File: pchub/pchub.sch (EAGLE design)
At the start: 73 parts, among them J6 2040210-1, J7 2040210-1, U1 SN74CBT16214DGGR, U10 FSUSB63UMX, U11 FSUSB63UMX, U12 FSUSB63UMX, U13 FSUSB63UMX, U14 FSUSB63UMX, U15 FSUSB63UMX, U16 FSUSB63UMX, U17 FSUSB63UMX, U18 FSUSB63UMX, U19 FSUSB63UMX, U2 SN74CBT16214DGGR, U20 FSUSB63UMX, U3 SN74CBT16214DGGR, U4 SN74CBT16214DGGR, U5 TMDS361BPAG, U6 TMDS361BPAG, U7 TMDS361BPAG, U8 TMDS361BPAG, U9 FSUSB63UMX, X1 USB, X10 USB, X11 USB, X12 USB, X13 USB, X2 USB, X3 USB, X4 USB, X5 USB, X6 USB, X7 USB, X8 USB, X9 USB

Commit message: m
,
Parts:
- added S17: (no value), SparkFun-Switches:SWITCH-SP3T-SMD
- added U$10, U$11, U$12, U$13, U$14, U$15, U$16, U$17, U$18, U$6, U$7, U$8, U$9: RJ45-8PTH, SparkFun:RJ45-8PTH
- added U21, U22: MAX4998ETIT, MAX4998ETIT:MAX4998ETIT
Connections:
- new net ETH1: U$10.1, U$11.1, U$12.1, U$13.1, U$14.1, U$15.1, U$16.1, U$17.1, U$18.1, U$6.1, U$7.1, U$8.1, U$9.1
- new net ETH2: U$10.2, U$11.2, U$12.2, U$13.2, U$14.2, U$15.2, U$16.2, U$17.2, U$18.2, U$6.2, U$7.2, U$8.2, U$9.2
- new net ETH3: U$10.3, U$11.3, U$12.3, U$13.3, U$14.3, U$15.3, U$16.3, U$17.3, U$18.3, U$6.3, U$7.3, U$8.3, U$9.3
- new net ETH4: U$10.4, U$11.4, U$12.4, U$13.4, U$14.4, U$15.4, U$16.4, U$17.4, U$18.4, U$6.4, U$7.4, U$8.4, U$9.4
- new net ETH5: U$10.5, U$11.5, U$12.5, U$13.5, U$14.5, U$15.5, U$16.5, U$17.5, U$18.5, U$6.5, U$7.5, U$8.5, U$9.5
- new net ETH6: U$10.6, U$11.6, U$12.6, U$13.6, U$14.6, U$15.6, U$16.6, U$17.6, U$18.6, U$6.6, U$7.6, U$8.6, U$9.6
- new net ETH7: U$10.7, U$11.7, U$12.7, U$13.7, U$14.7, U$15.7, U$16.7, U$17.7, U$18.7, U$6.7, U$7.7, U$8.7, U$9.7
- new net ETH8: U$10.8, U$11.8, U$12.8, U$13.8, U$14.8, U$15.8, U$16.8, U$17.8, U$18.8, U$6.8, U$7.8, U$8.8, U$9.8
- net HDMIGND: now also J1SHIELD.SHIELD
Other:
- note added: "ETHERNET"
- moved on the sheet: J1G$1, J1SHIELD, J6, J7

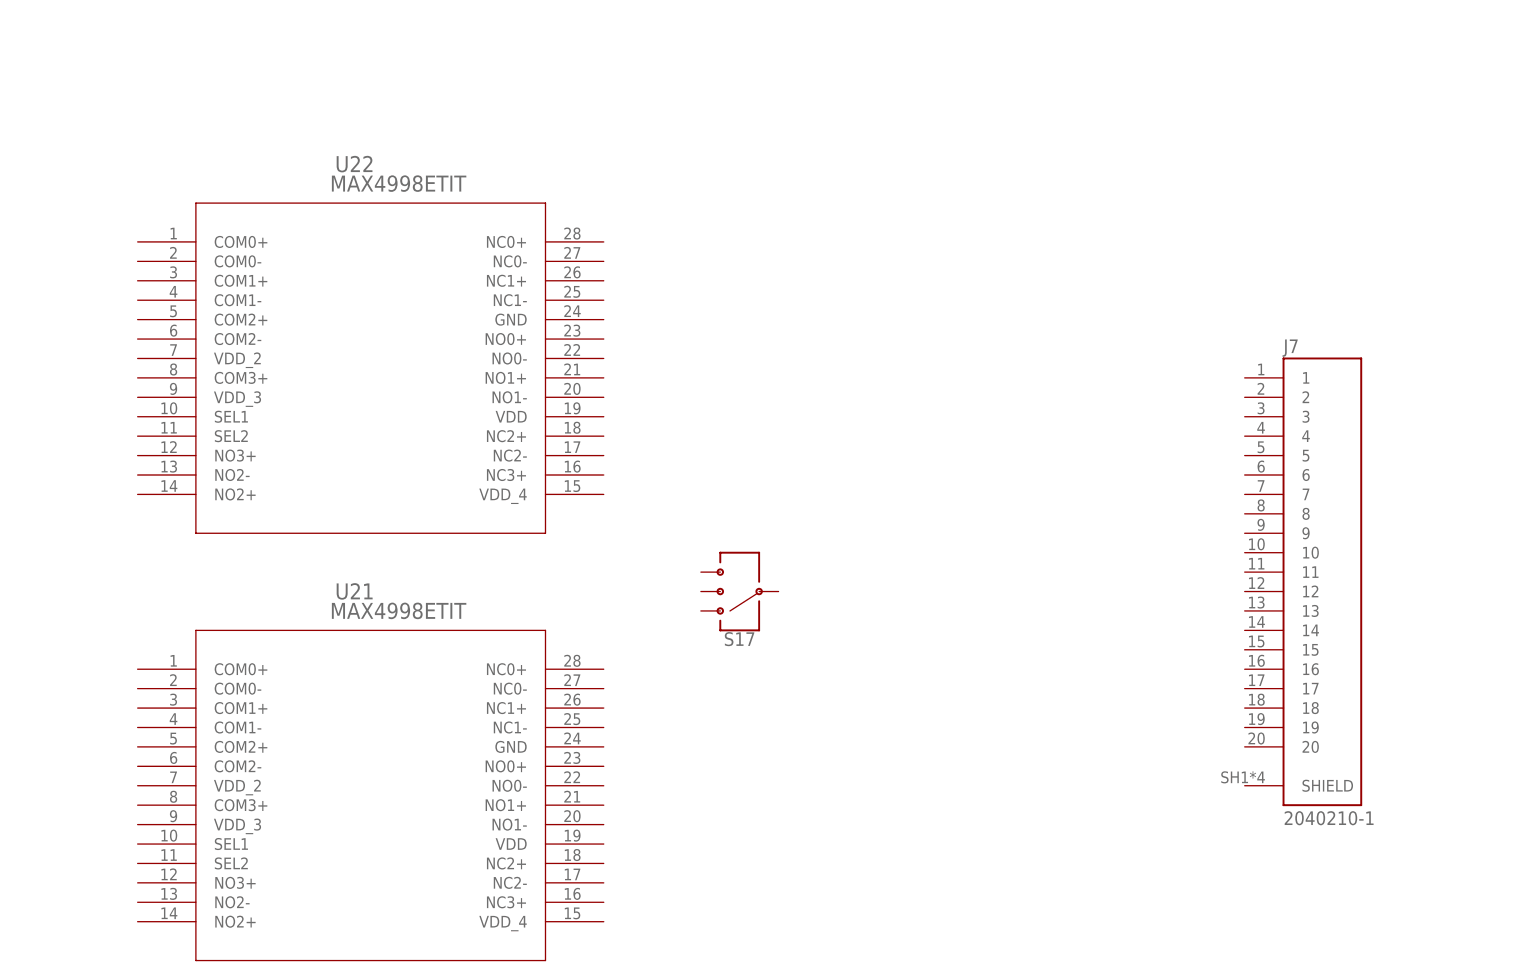
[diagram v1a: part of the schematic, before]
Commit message: sd
asdsa
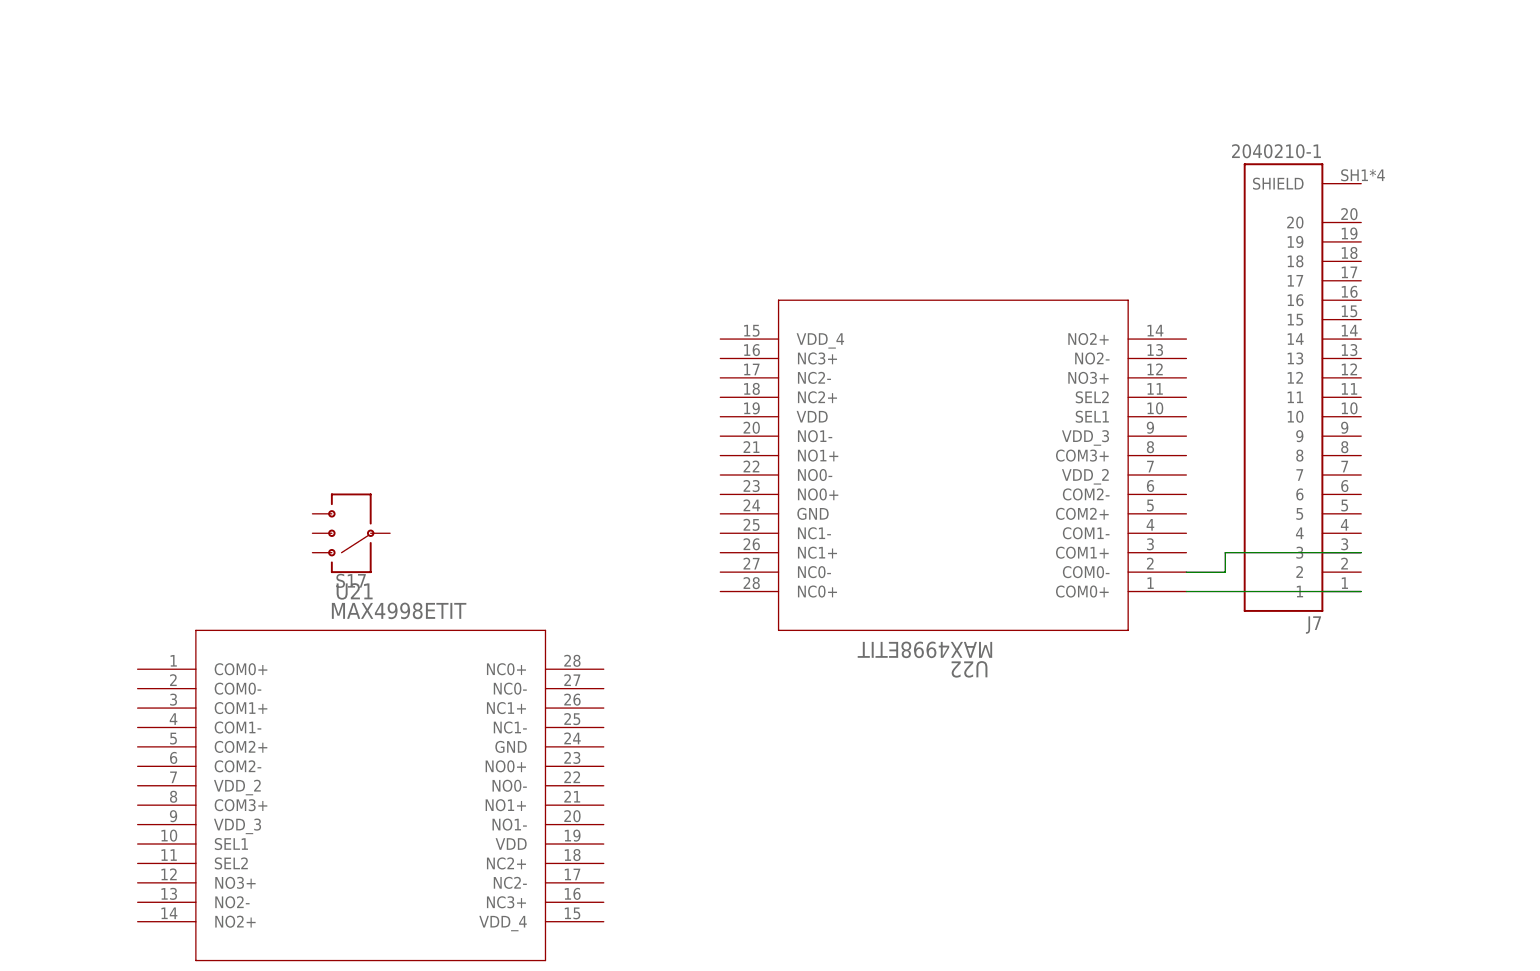
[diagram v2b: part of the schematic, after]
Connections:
- new net N$130: J7.1, U22.COM0+
- new net N$131: J7.3, U22.COM0-
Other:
- moved on the sheet: J7, S17, U22
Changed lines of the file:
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@@
 <layer number="59" name="tCarbon" color="7" fill="1" visible="no" active="no"/>
 <layer number="60" name="bCarbon" color="7" fill="1" visible="no" active="no"/>
-<layer number="88" name="SimResults" color="9" fill="1" visible="yes" active="yes"/>
+<layer number="88" name="SimResults" color="9" fill="1" visible="no" active="yes"/>
 <layer number="89" name="SimProbes" color="9" fill="1" visible="yes" active="yes"/>
 <layer number="90" name="Modules" color="5" fill="1" visible="yes" active="yes"/>
@@
 <instance part="D12" gate="G$1" x="-431.8" y="190.5" rot="R270"/>
 <instance part="J6" gate="G$1" x="-601.98" y="231.14"/>
-<instance part="J7" gate="G$1" x="-213.36" y="-119.38"/>
+<instance part="J7" gate="G$1" x="-218.44" y="-91.44" rot="R180"/>
 <instance part="U$6" gate="G$1" x="-601.98" y="287.02"/>
 <instance part="U$11" gate="G$1" x="-317.5" y="127"/>
@@
 <instance part="U$18" gate="G$1" x="-424.18" y="30.48"/>
 <instance part="U21" gate="A" x="-368.3" y="-129.54"/>
-<instance part="U22" gate="A" x="-368.3" y="-73.66"/>
-<instance part="S17" gate="G$1" x="-289.56" y="-119.38" rot="R180"/>
+<instance part="U22" gate="A" x="-231.14" y="-119.38" rot="R180"/>
+<instance part="S17" gate="G$1" x="-340.36" y="-111.76" rot="R180"/>
 </instances>
 <busses>
@@
 </segment>
 </net>
+<net name="N$130" class="0">
+<segment>
+<pinref part="U22" gate="A" pin="COM0+"/>
+<pinref part="J7" gate="G$1" pin="1"/>
+<wire x1="-231.14" y1="-119.38" x2="-208.28" y2="-119.38" width="0.1524" layer="91"/>
+</segment>
+</net>
+<net name="N$131" class="0">
+<segment>
+<pinref part="J7" gate="G$1" pin="3"/>
+<wire x1="-208.28" y1="-114.3" x2="-226.06" y2="-114.3" width="0.1524" layer="91"/>
+<wire x1="-226.06" y1="-114.3" x2="-226.06" y2="-116.84" width="0.1524" layer="91"/>
+<pinref part="U22" gate="A" pin="COM0-"/>
+<wire x1="-226.06" y1="-116.84" x2="-231.14" y2="-116.84" width="0.1524" layer="91"/>
+</segment>
+</net>

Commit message: s
s
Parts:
- removed U$10, U$11, U$12, U$13, U$14, U$15, U$16, U$17, U$18, U$7, U$8, U$9: RJ45-8PTH, SparkFun:RJ45-8PTH
- added J10, J8, J9: 2040210-1, 2040210-1:2040210-1
- added J11, J12: AUDIO_JACK_TRRSSMD_RA, SparkFun-Connectors:AUDIO_JACK_TRRSSMD_RA
- added S18, S19, S20: (no value), SparkFun-Switches:SWITCH-SP3T-SMD
- added U$19, U$20, U$21, U$22, U$23, U$24, U$25, U$26, U$27, U$28, U$29, U$30: RJ45-8PTH, SparkFun:RJ45-8PTH
- added U23, U24, U25, U26, U27, U28: SN74CBT16214DGGR, SN74CBT16214DGGR:SN74CBT16214DGGR
- U21, U22: value MAX4998ETIT -> SN74CBT16214DGGR; device MAX4998ETIT:MAX4998ETIT -> SN74CBT16214DGGR:SN74CBT16214DGGR
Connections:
- new net B$1: U21.10A, U23.10A, U25.10A, U27.10A
- new net B$2: U21.11A, U23.11A, U25.11A, U27.11A
- new net N$143: J7.3, U21.3A
- new net N$144: J7.4, U21.4A
- new net N$145: J7.5, U21.5A
- new net N$146: J7.6, U21.6A
- new net N$147: J7.7, U21.7A
- new net N$148: J7.8, U21.8A
- new net N$149: J7.9, U21.9A
- new net N$150: J7.10
- new net N$151: J7.11
- new net N$152: J7.12, U21.12A
- new net N$153: J7.13, U22.1A
- new net N$154: J7.14, U22.2A
- new net N$155: J7.15, U22.3A
- new net N$156: J7.16, U22.4A
- new net N$157: J7.17, U22.5A
- new net N$158: J7.18, U22.6A
- new net N$159: J7.19, U22.7A
- new net N$160: J7.SHIELD, U22.9A
- new net N$161: J8.1, U23.1A
- new net N$162: J8.2, U23.2A
- new net N$163: J7.20, U22.8A
- new net N$164: J8.3, U23.3A
- new net N$165: J8.4, U23.4A
- new net N$166: J8.5, U23.5A
- new net N$167: J8.6, U23.6A
- new net N$168: J8.7, U23.7A
- new net N$169: J8.8, U23.8A
- new net N$170: J8.9, U23.9A
- new net N$171: J8.10
- new net N$172: J8.11
- new net N$173: J8.12, U23.12A
- new net N$174: J8.13, U24.1A
- new net N$175: J8.14, U24.2A
- new net N$176: J8.15, U24.3A
- new net N$177: J8.16, U24.4A
- new net N$178: J8.17, U24.5A
- new net N$179: J8.18, U24.6A
- new net N$180: J8.19, U24.7A
- new net N$181: J8.SHIELD, U24.9A
- new net N$182: J8.20, U24.8A
- new net N$183: J9.1, U25.1A
- new net N$184: J9.2, U25.2A
- new net N$185: J9.3, U25.3A
- new net N$186: J9.4, U25.4A
- new net N$187: J9.5, U25.5A
- new net N$188: J9.6, U25.6A
- new net N$189: J9.7, U25.7A
- new net N$190: J9.8, U25.8A
- new net N$191: J9.9, U25.9A
- new net N$192: J9.10
- new net N$193: J9.11
- new net N$194: J9.12, U25.12A
- new net N$195: J9.13, U26.1A
- new net N$196: J9.14, U26.2A
- new net N$197: J9.15, U26.3A
- new net N$198: J9.16, U26.4A
- new net N$199: J9.17, U26.5A
- new net N$200: J9.18, U26.6A
- new net N$201: J9.19, U26.7A
- new net N$202: J9.SHIELD, U26.9A
- new net N$203: J9.20, U26.8A
- new net N$204: J10.1, U27.1A
- new net N$205: J10.2, U27.2A
- new net N$206: J10.3, U27.3A
- new net N$207: J10.4, U27.4A
- new net N$208: J10.5, U27.5A
- new net N$209: J10.6, U27.6A
- new net N$210: J10.7, U27.7A
- new net N$211: J10.8, U27.8A
- new net N$212: J10.9, U27.9A
- new net N$213: J10.10
- new net N$214: J10.11
- new net N$215: J10.12, U27.12A
- new net N$216: J10.13, U28.1A
- new net N$217: J10.14, U28.2A
- new net N$218: J10.15, U28.3A
- new net N$219: J10.16, U28.4A
- new net N$220: J10.17, U28.5A
- new net N$221: J10.18, U28.6A
- new net N$222: J10.19, U28.7A
- new net N$223: J10.SHIELD, U28.9A
- new net N$224: J10.20, U28.8A
- new net PC1A1: J11.RING2, J12.RING2
- new net PC1A2: J11.TIP, J12.TIP
- new net PC1A3: J11.RING1, J12.RING1
- new net PC1A4: J11.EARTH, J12.EARTH
- new net PC1DP1: J6.1, U21.1B1, U23.1B1, U25.1B1, U27.1B1
- new net PC1DP10: J6.10, U21.10B1, U23.10B1, U25.10B1, U27.10B1
- new net PC1DP11: J6.11, U21.11B1, U23.11B1, U25.11B1, U27.11B1
- new net PC1DP12: J6.12, U21.12B1, U23.12B1, U25.12B1, U27.12B1
- new net PC1DP13: J6.13, U22.1B1, U24.1B1, U26.1B1, U28.1B1
- new net PC1DP14: J6.14, U22.2B1, U24.2B1, U26.2B1, U28.2B1
- new net PC1DP15: J6.15, U22.3B1, U24.3B1, U26.3B1, U28.3B1
- new net PC1DP16: J6.16, U22.4B1, U24.4B1, U26.4B1, U28.4B1
- new net PC1DP17: J6.17, U22.5B1, U24.5B1, U26.5B1, U28.5B1
- new net PC1DP18: J6.18, U22.6B1, U24.6B1, U26.6B1, U28.6B1
- new net PC1DP19: J6.19, U22.7B1, U24.7B1, U26.7B1, U28.7B1
- new net PC1DP2: J6.2, U21.2B1, U23.2B1, U25.2B1, U27.2B1
- new net PC1DP20: J6.20, U22.8B1, U24.8B1, U26.8B1, U28.8B1
- new net PC1DP3: J6.3, U21.3B1, U23.3B1, U25.3B1, U27.3B1
- new net PC1DP4: J6.4, U21.4B1, U23.4B1, U25.4B1, U27.4B1
- new net PC1DP5: J6.5, U21.5B1, U23.5B1, U25.5B1, U27.5B1
- new net PC1DP6: J6.6, U21.6B1, U23.6B1, U25.6B1, U27.6B1
- new net PC1DP7: J6.7, U21.7B1, U23.7B1, U25.7B1, U27.7B1
- new net PC1DP8: J6.8, U21.8B1, U23.8B1, U25.8B1, U27.8B1
- new net PC1DP9: J6.9, U21.9B1, U23.9B1, U25.9B1, U27.9B1
- new net PC1DPS: J6.SHIELD, U22.9B1, U24.9B1, U26.9B1, U28.9B1
- new net PC2DP1: U21.1B2, U23.1B2, U25.1B2, U27.1B2
- new net PC2DP10: U21.10B2, U23.10B2, U25.10B2, U27.10B2
- new net PC2DP11: U21.11B2, U23.11B2, U25.11B2, U27.11B2
- new net PC2DP12: U21.12B2, U23.12B2, U25.12B2, U27.12B2
- new net PC2DP13: U22.1B2, U24.1B2, U26.1B2, U28.1B2
- new net PC2DP14: U22.2B2, U24.2B2, U26.2B2, U28.2B2
- new net PC2DP15: U22.3B2, U24.3B2, U26.3B2, U28.3B2
- new net PC2DP16: U22.4B2, U24.4B2, U26.4B2, U28.4B2
- new net PC2DP17: U22.5B2, U24.5B2, U26.5B2, U28.5B2
- new net PC2DP18: U22.6B2, U24.6B2, U26.6B2, U28.6B2
- new net PC2DP19: U22.7B2, U24.7B2, U26.7B2, U28.7B2
- new net PC2DP2: U21.2B2, U23.2B2, U25.2B2, U27.2B2
- new net PC2DP20: U22.8B2, U24.8B2, U26.8B2, U28.8B2
- new net PC2DP3: U21.3B2, U23.3B2, U25.3B2, U27.3B2
- new net PC2DP4: U21.4B2, U23.4B2, U25.4B2, U27.4B2
- new net PC2DP5: U21.5B2, U23.5B2, U25.5B2, U27.5B2
- new net PC2DP6: U21.6B2, U23.6B2, U25.6B2, U27.6B2
- new net PC2DP7: U21.7B2, U23.7B2, U25.7B2, U27.7B2
- new net PC2DP8: U21.8B2, U23.8B2, U25.8B2, U27.8B2
- new net PC2DP9: U21.9B2, U23.9B2, U25.9B2, U27.9B2
- new net PC2DPS: U22.9B2, U24.9B2, U26.9B2, U28.9B2
- new net PC3DP1: U21.1B3, U23.1B3, U25.1B3, U27.1B3
- new net PC3DP10: U21.10B3, U23.10B3, U25.10B3, U27.10B3
- new net PC3DP11: U21.11B3, U23.11B3, U25.11B3, U27.11B3
- new net PC3DP12: U21.12B3, U23.12B3, U25.12B3, U27.12B3
- new net PC3DP13: U22.1B3, U24.1B3, U26.1B3, U28.1B3
- new net PC3DP14: U22.2B3, U24.2B3, U26.2B3, U28.2B3
- new net PC3DP15: U22.3B3, U24.3B3, U26.3B3, U28.3B3
- new net PC3DP16: U22.4B3, U24.4B3, U26.4B3, U28.4B3
- new net PC3DP17: U22.5B3, U24.5B3, U26.5B3, U28.5B3
- new net PC3DP18: U22.6B3, U24.6B3, U26.6B3, U28.6B3
- new net PC3DP19: U22.7B3, U24.7B3, U26.7B3, U28.7B3
- new net PC3DP2: U21.2B3, U23.2B3, U25.2B3, U27.2B3
- new net PC3DP20: U22.8B3, U24.8B3, U26.8B3, U28.8B3
- new net PC3DP3: U21.3B3, U23.3B3, U25.3B3, U27.3B3
- new net PC3DP4: U21.4B3, U23.4B3, U25.4B3, U27.4B3
- new net PC3DP5: U21.5B3, U23.5B3, U25.5B3, U27.5B3
- new net PC3DP6: U21.6B3, U23.6B3, U25.6B3, U27.6B3
- new net PC3DP7: U21.7B3, U23.7B3, U25.7B3, U27.7B3
- new net PC3DP8: U21.8B3, U23.8B3, U25.8B3, U27.8B3
- new net PC3DP9: U21.9B3, U23.9B3, U25.9B3, U27.9B3
- new net PC3DPS: U22.9B3, U24.9B3, U26.9B3, U28.9B3
- net ETH1: now also U$19.1, U$20.1, U$21.1, U$22.1, U$23.1, U$24.1, U$25.1, U$26.1, U$27.1, U$28.1, U$29.1, U$30.1; no longer U$10.1, U$11.1, U$12.1, U$13.1, U$14.1, U$15.1, U$16.1, U$17.1, U$18.1, U$7.1, U$8.1, U$9.1
- net ETH2: now also U$19.2, U$20.2, U$21.2, U$22.2, U$23.2, U$24.2, U$25.2, U$26.2, U$27.2, U$28.2, U$29.2, U$30.2; no longer U$10.2, U$11.2, U$12.2, U$13.2, U$14.2, U$15.2, U$16.2, U$17.2, U$18.2, U$7.2, U$8.2, U$9.2
- net ETH3: now also U$19.3, U$20.3, U$21.3, U$22.3, U$23.3, U$24.3, U$25.3, U$26.3, U$27.3, U$28.3, U$29.3, U$30.3; no longer U$10.3, U$11.3, U$12.3, U$13.3, U$14.3, U$15.3, U$16.3, U$17.3, U$18.3, U$7.3, U$8.3, U$9.3
- net ETH4: now also U$19.4, U$20.4, U$21.4, U$22.4, U$23.4, U$24.4, U$25.4, U$26.4, U$27.4, U$28.4, U$29.4, U$30.4; no longer U$10.4, U$11.4, U$12.4, U$13.4, U$14.4, U$15.4, U$16.4, U$17.4, U$18.4, U$7.4, U$8.4, U$9.4
- net ETH5: now also U$19.5, U$20.5, U$21.5, U$22.5, U$23.5, U$24.5, U$25.5, U$26.5, U$27.5, U$28.5, U$29.5, U$30.5; no longer U$10.5, U$11.5, U$12.5, U$13.5, U$14.5, U$15.5, U$16.5, U$17.5, U$18.5, U$7.5, U$8.5, U$9.5
- net ETH6: now also U$19.6, U$20.6, U$21.6, U$22.6, U$23.6, U$24.6, U$25.6, U$26.6, U$27.6, U$28.6, U$29.6, U$30.6; no longer U$10.6, U$11.6, U$12.6, U$13.6, U$14.6, U$15.6, U$16.6, U$17.6, U$18.6, U$7.6, U$8.6, U$9.6
- net ETH7: now also U$19.7, U$20.7, U$21.7, U$22.7, U$23.7, U$24.7, U$25.7, U$26.7, U$27.7, U$28.7, U$29.7, U$30.7; no longer U$10.7, U$11.7, U$12.7, U$13.7, U$14.7, U$15.7, U$16.7, U$17.7, U$18.7, U$7.7, U$8.7, U$9.7
- net ETH8: now also U$19.8, U$20.8, U$21.8, U$22.8, U$23.8, U$24.8, U$25.8, U$26.8, U$27.8, U$28.8, U$29.8, U$30.8; no longer U$10.8, U$11.8, U$12.8, U$13.8, U$14.8, U$15.8, U$16.8, U$17.8, U$18.8, U$7.8, U$8.8, U$9.8
- net N$130: now also U21.1A; no longer U22.COM0+
- net N$131: now also J7.2, U21.2A; no longer J7.3, U22.COM0-
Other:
- note added: "DP"
- moved on the sheet: J1G$1, J1SHIELD, J6, J7, S17, U$6
